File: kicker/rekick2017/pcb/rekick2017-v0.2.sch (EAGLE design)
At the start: 184 parts, among them IC1 SN74LVC1G02DBVR, IC2 4043D, IC3 LM1117, IC4 MCP602-I/SN, P1 39-30-06_S, P2 39-30-08_S, Q1 16MHz, Q2 IKW40N120T2FKSA1, Q3 PSMN7R8-120PS, Q4 PSMN7R8-120PS, Q5 IPD90P04P4L, Q6 IRF840, T1 BC859, T5 IRLML6344TRPBF, U1 TXB0108PWR, U2 R-7805, U3 R-7812, U4 R-7805, U5 ADUM4190BRIZ

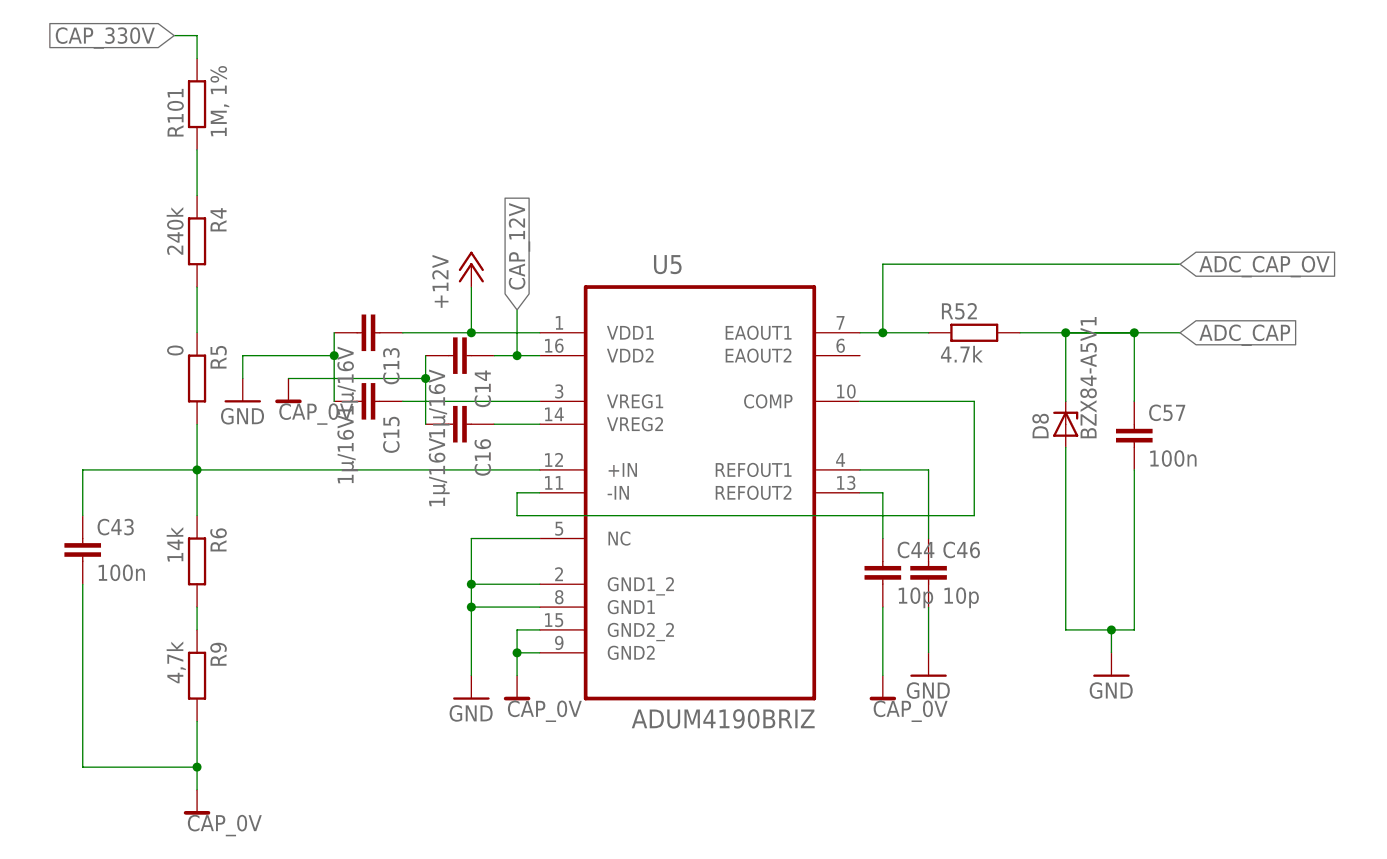
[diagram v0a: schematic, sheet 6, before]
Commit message: rekick2017 0.2 (TODO: finish layout)
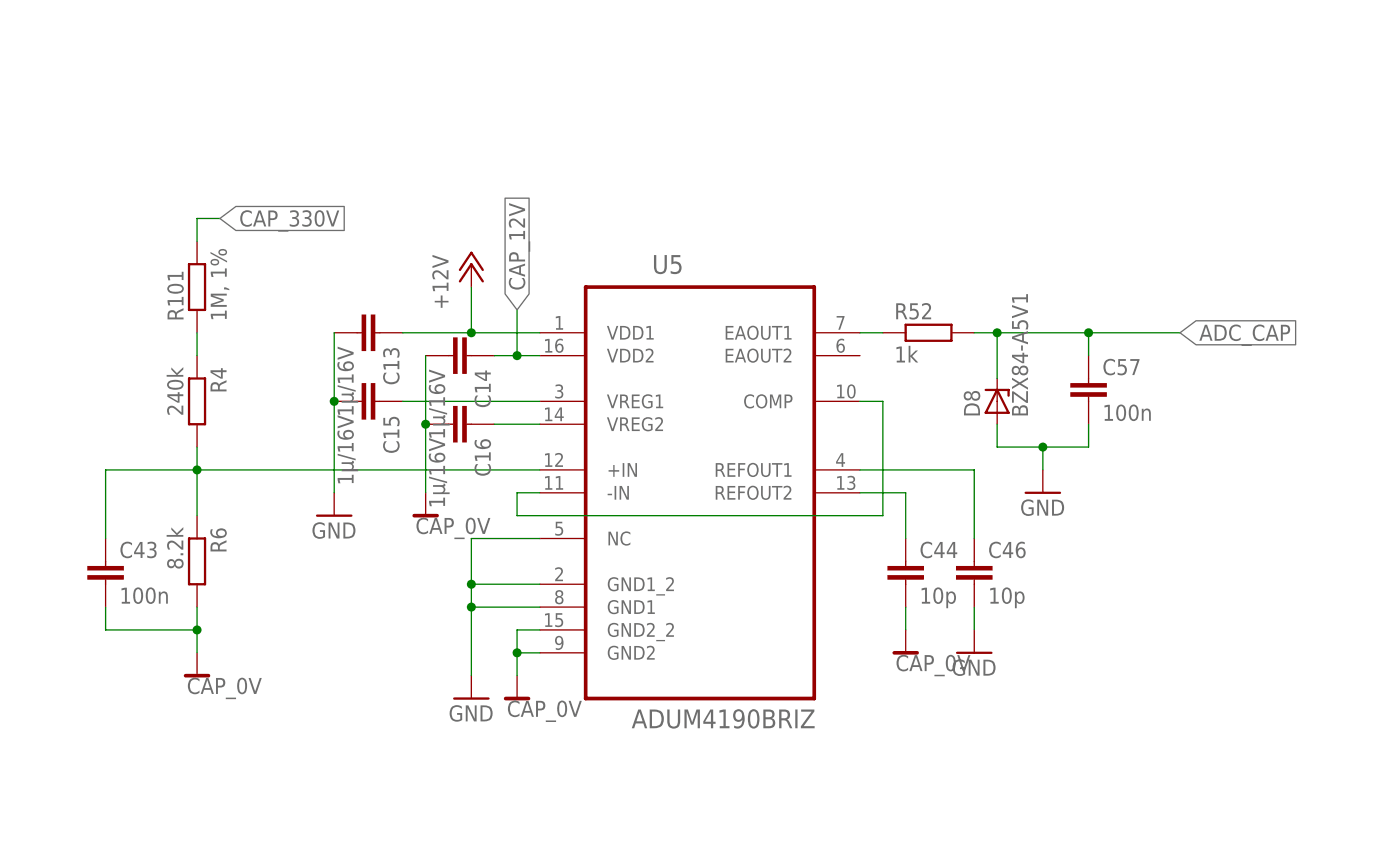
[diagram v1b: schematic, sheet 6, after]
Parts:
- removed R9: 4,7k, rcl:R-EU_R0805
- added C22: 100n, rcl:C-EUC0603
- R3: value 4.7k -> 43k
- R35: value 100k -> 33k
- R5: value 0 -> 1k
- R52: value 4.7k -> 1k
- R6: value 14k -> 8.2k
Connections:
- removed net ADC_CAP_OV: IC4B.+IN, R52.1, U5.EAOUT1
- removed net FB_TRIG_LVL: C20.1, IC4A.-IN, R3.1, R35.2
- removed net N$27: R6.2, R9.1
- new net TRIG_LVL_FB: C20.1, C22.2, IC4A.-IN, R35.2, R5.1
- new net TRIG_LVL_OV: C22.1, IC4B.-IN, R3.1, R5.2
- net +5V/3: no longer IC4B.-IN
- net ADC_CAP: now also IC4B.+IN
- net CAP_0V: now also R6.2; no longer R9.2
- net N$14: now also R4.2; no longer R5.2
- net N$15: now also R52.1, U5.EAOUT1; no longer R4.2, R5.1
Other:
- moved on the sheet: C20, C43, C44, C46, C57, D8, IC4A, IC4B, R101, R33, R35, R4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
